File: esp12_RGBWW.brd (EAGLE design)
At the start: 53 x 47 mm, 37 parts, among them Q1 AOD2910SMD, Q2 AOD2910SMD, Q3 AOD2910SMD, Q4 AOD2910SMD, Q5 AOD2910SMD, U1 TPS5410DR

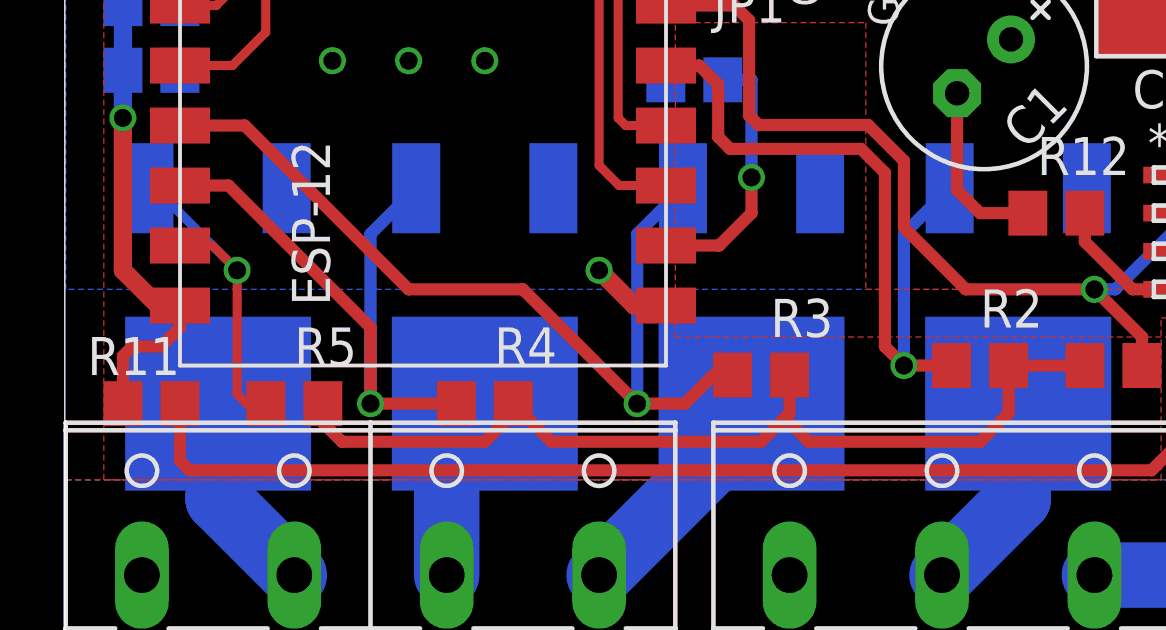
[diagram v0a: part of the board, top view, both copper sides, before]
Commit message: final production version
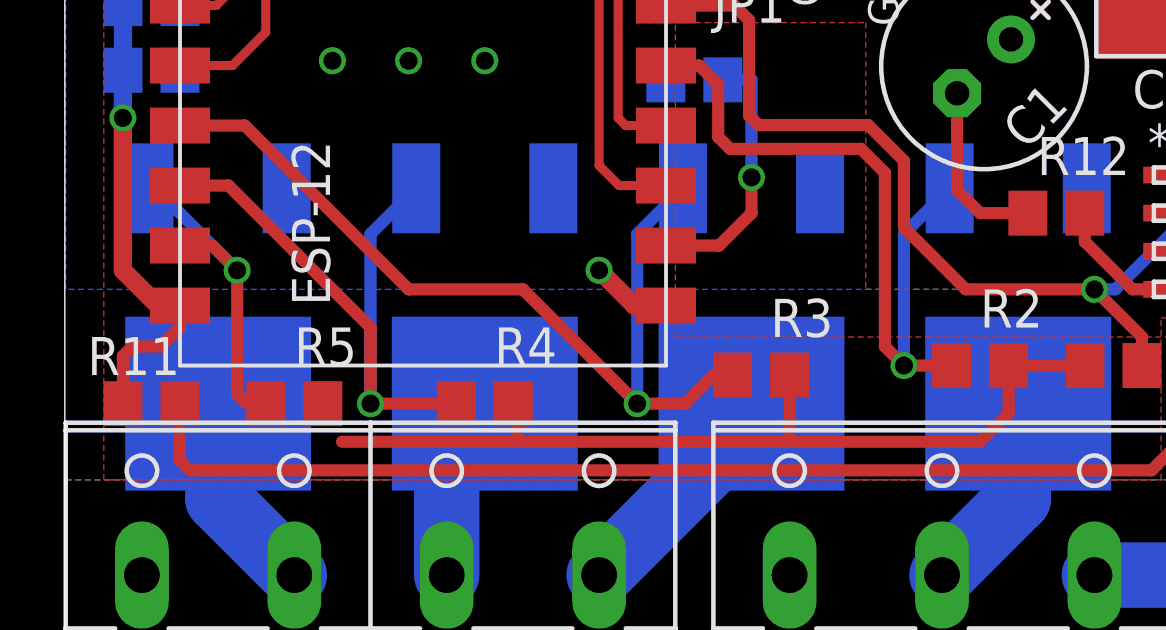
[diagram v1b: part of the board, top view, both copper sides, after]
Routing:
- net GND: track 58.4 -> 57.1 mm
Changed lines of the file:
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@@
 <wire x1="22.86" y1="27.94" x2="22.225" y2="27.305" width="0.254" layer="25"/>
 <wire x1="25.4" y1="27.94" x2="26.035" y2="28.575" width="0.254" layer="25"/>
-<text x="18.415" y="29.845" size="1.016" layer="26" rot="MR0">Lightinator 3, brought to you
+<text x="18.415" y="29.845" size="0.8128" layer="26" font="vector" rot="MR0">Lightinator 3, brought to you
 by the fhem community
 http://forum.fhem.de</text>
@@
 <contactref element="VCC" pad="2"/>
 <via x="16.51" y="14.605" extent="1-16" drill="0.6"/>
-<wire x1="14.92" y1="8.89" x2="13.65" y2="10.16" width="0.4064" layer="1"/>
-<wire x1="13.65" y1="10.16" x2="13.65" y2="9.84" width="0.4064" layer="1"/>
-<wire x1="13.65" y1="9.84" x2="12.7" y2="8.89" width="0.4064" layer="1"/>
 <wire x1="16.51" y1="14.605" x2="17.685" y2="13.43" width="0.6096" layer="1"/>
 <wire x1="17.685" y1="13.43" x2="18.74" y2="13.43" width="0.6096" layer="1"/>
@@
 <wire x1="45.4025" y1="31.75" x2="45.4025" y2="32.995" width="0.3048" layer="1"/>
 <wire x1="45.4025" y1="32.995" x2="45.3775" y2="32.7025" width="0.3048" layer="1"/>
-<wire x1="12.7" y1="8.89" x2="7.9375" y2="8.89" width="0.4064" layer="1"/>
-<wire x1="7.9375" y1="8.89" x2="7.3" y2="9.5275" width="0.4064" layer="1"/>
-<wire x1="7.3" y1="9.5275" x2="7.3" y2="10.16" width="0.4064" layer="1"/>
 <wire x1="26.9625" y1="32.7025" x2="25.4" y2="32.7025" width="0.3048" layer="1"/>
 <wire x1="25.4" y1="32.7025" x2="25.0825" y2="33.02" width="0.3048" layer="1"/>
@@
 <vertex x="0" y="7.62"/>
 </polygon>
-<wire x1="14.92" y1="8.89" x2="21.9075" y2="8.89" width="0.4064" layer="1"/>
-<wire x1="21.9075" y1="8.89" x2="22.70125" y2="9.68375" width="0.4064" layer="1"/>
-<wire x1="22.70125" y1="9.68375" x2="22.8575" y2="9.84" width="0.4064" layer="1"/>
-<wire x1="22.8575" y1="9.84" x2="22.8575" y2="11.1125" width="0.4064" layer="1"/>
+<wire x1="7.9375" y1="8.89" x2="13.81125" y2="8.89" width="0.4064" layer="1"/>
+<wire x1="13.81125" y1="8.89" x2="22.86" y2="8.89" width="0.4064" layer="1"/>
 <wire x1="30.1625" y1="11.4275" x2="30.1625" y2="9.8425" width="0.4064" layer="1"/>
 <wire x1="30.1625" y1="9.8425" x2="29.21" y2="8.89" width="0.4064" layer="1"/>
-<wire x1="29.21" y1="8.89" x2="23.495" y2="8.89" width="0.4064" layer="1"/>
-<wire x1="23.495" y1="8.89" x2="22.70125" y2="9.68375" width="0.4064" layer="1"/>
+<wire x1="29.21" y1="8.89" x2="22.86" y2="8.89" width="0.4064" layer="1"/>
 <contactref element="PRG" pad="2"/>
 <contactref element="JP1" pad="6"/>
@@
 <via x="10.16" y="21.59" extent="1-16" drill="0.6" shape="octagon"/>
 <via x="7.62" y="21.59" extent="1-16" drill="0.6" shape="octagon"/>
+<wire x1="13.65" y1="10.16" x2="13.81125" y2="10.16" width="0.4064" layer="1"/>
+<wire x1="13.81125" y1="10.16" x2="13.81125" y2="8.89" width="0.4064" layer="1"/>
+<wire x1="22.8575" y1="11.1125" x2="22.86" y2="11.1125" width="0.4064" layer="1"/>
+<wire x1="22.86" y1="11.1125" x2="22.86" y2="8.89" width="0.4064" layer="1"/>
 </signal>
 <signal name="RST_S" class="5">
@@
 <wire x1="1.524" y1="17.34" x2="0.83" y2="17.34" width="0.4064" layer="16"/>
 <wire x1="2.54" y1="15.43" x2="3.62" y2="15.43" width="0.3048" layer="1"/>
-<wire x1="3.62" y1="15.43" x2="4.445" y2="14.605" width="0.3048" layer="1"/>
-<wire x1="4.445" y1="14.605" x2="4.445" y2="10.4775" width="0.3048" layer="1"/>
+<wire x1="3.62" y1="15.43" x2="4.445" y2="14.605" width="0.4064" layer="1"/>
+<wire x1="4.445" y1="14.605" x2="4.445" y2="10.4775" width="0.4064" layer="1"/>
 <wire x1="1.524" y1="17.34" x2="1.71" y2="17.34" width="0.3048" layer="16"/>
-<wire x1="1.71" y1="17.34" x2="4.445" y2="14.605" width="0.3048" layer="16"/>
-<wire x1="4.445" y1="10.4775" x2="4.7625" y2="10.16" width="0.3048" layer="1"/>
+<wire x1="1.71" y1="17.34" x2="4.445" y2="14.605" width="0.4064" layer="16"/>
+<wire x1="4.445" y1="10.4775" x2="4.7625" y2="10.16" width="0.4064" layer="1"/>
 <wire x1="4.7625" y1="10.16" x2="5.4" y2="10.16" width="0.3048" layer="1"/>
 </signal>
